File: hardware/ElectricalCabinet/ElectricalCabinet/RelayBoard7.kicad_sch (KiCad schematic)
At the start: 0 parts

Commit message: Further wiring updates
Populated 6100 Bus
Corrected number of relay boards
Added 110v outputs to relay boards and noted light positon
Uploaded light scheme to documents folder
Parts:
- added C7: 0.1uF, Capacitor_SMD:C_0805_2012Metric, symbol Device:C
- added D49, D50, D51, D52, D53, D54, D55, D56: LED, LED_SMD:LED_0805_2012Metric, symbol Device:LED
- added J14: Screw_Terminal_01x06, TerminalBlock:TerminalBlock_MaiXu_MX126-5.0-06P_1x06_P5.00mm, symbol Connector:Screw_Terminal_01x06
- added J15: Screw_Terminal_01x09, TerminalBlock:TerminalBlock_MaiXu_MX126-5.0-09P_1x09_P5.00mm, symbol Connector:Screw_Terminal_01x09
- added K49, K50, K51, K52, K53, K54, K55, K56: G3MB-202P DC5, TrafficLightLibrary:G3MB_202P_DC5, symbol TrafficLightLibrary:G3MB-202P_DC5
- added R49, R50, R51, R52, R53, R54, R55, R56: 1kΩ, Resistor_SMD:R_0805_2012Metric, symbol Device:R
- added U8: TPIC6B595N, TrafficLightLibrary:TPIC6B595N, symbol TrafficLightLibrary:TPIC6B595N
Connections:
- new net: D51.1 (K), R51.1
- new net: K51.4, R51.2, U8.6 (DRAIN2)
- new net: J15.9 (Pin_9), K49.1, K50.1, K51.1, K52.1, K53.1, K54.1, K55.1, K56.1
- new net: J15.8 (Pin_8), K56.2
- new net: D49.2 (A), D50.2 (A), D51.2 (A), D52.2 (A), D53.2 (A), D54.2 (A), D55.2 (A), D56.2 (A), K49.3, K50.3, K51.3, K52.3, K53.3, K54.3, K55.3, K56.3
- new net: K56.4, R56.2, U8.17 (DRAIN7)
- new net: D50.1 (K), R50.1
- new net: J15.1 (Pin_1), K49.2
- new net: K49.4, R49.2, U8.4 (DRAIN0)
- new net: D52.1 (K), R52.1
- new net: J15.2 (Pin_2), K50.2
- new net: K50.4, R50.2, U8.5 (DRAIN1)
- new net: J15.3 (Pin_3), K51.2
- new net: J15.4 (Pin_4), K52.2
- new net: J15.5 (Pin_5), K53.2
- new net: J15.6 (Pin_6), K54.2
- new net: J15.7 (Pin_7), K55.2
- new net: C7.1, J14.2 (Pin_2), U8.10 (GND), U8.11 (GND), U8.19 (GND), U8.9 (~{G})
- new net: C7.2, J14.6 (Pin_6), U8.2 (VCC), U8.8 (~{SRCLR})
- new net: D55.1 (K), R55.1
- new net: D53.1 (K), R53.1
- new net: K52.4, R52.2, U8.7 (DRAIN3)
- new net: K55.4, R55.2, U8.16 (DRAIN6)
- new net: D54.1 (K), R54.1
- new net: K54.4, R54.2, U8.15 (DRAIN5)
- new net: J14.1 (Pin_1), U8.18 (SEROUT)
- new net: J14.3 (Pin_3), U8.13 (SRCK)
- new net: J14.4 (Pin_4), U8.12 (RCK)
- new net: D49.1 (K), R49.1
- new net: K53.4, R53.2, U8.14 (DRAIN4)
- new net: D56.1 (K), R56.1
- new net SERIN: J14.5 (Pin_5), U8.3 (SERIN)
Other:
- note added: "RELAY MODULE 7"

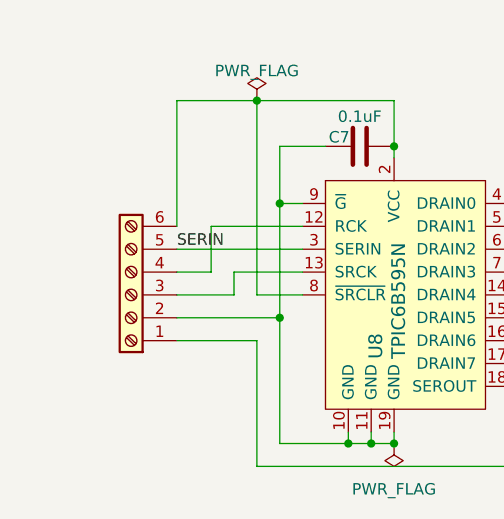
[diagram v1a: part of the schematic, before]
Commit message: Electrical Cabinet done
Electrical Cabinet done, let me know if there are any changes or mistakes.
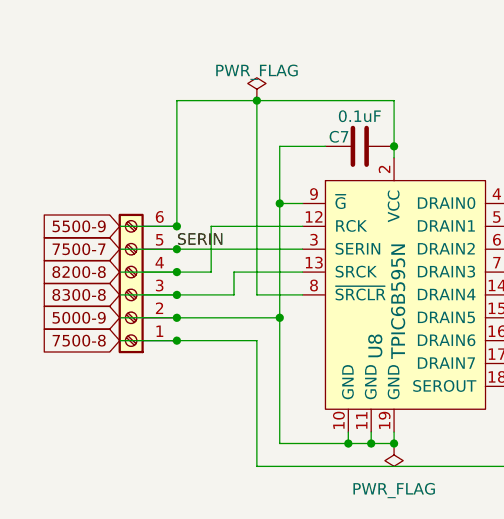
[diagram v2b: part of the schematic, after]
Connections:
- net 5000-9: now reaches C7.1, J14.2 (Pin_2), U8.10 (GND), U8.11 (GND), U8.19 (GND), U8.9 (~{G})
- net 5500-9: now reaches C7.2, J14.6 (Pin_6), U8.2 (VCC), U8.8 (~{SRCLR})
- net 7500-8: now reaches J14.1 (Pin_1), U8.18 (SEROUT)
- net 8300-8: now reaches J14.3 (Pin_3), U8.13 (SRCK)
- net 8200-8: now reaches J14.4 (Pin_4), U8.12 (RCK)
- net SERIN renamed 7500-7
